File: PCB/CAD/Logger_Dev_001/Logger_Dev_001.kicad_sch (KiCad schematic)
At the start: 11 parts, among them U2 ESP32-C6-WROOM-1

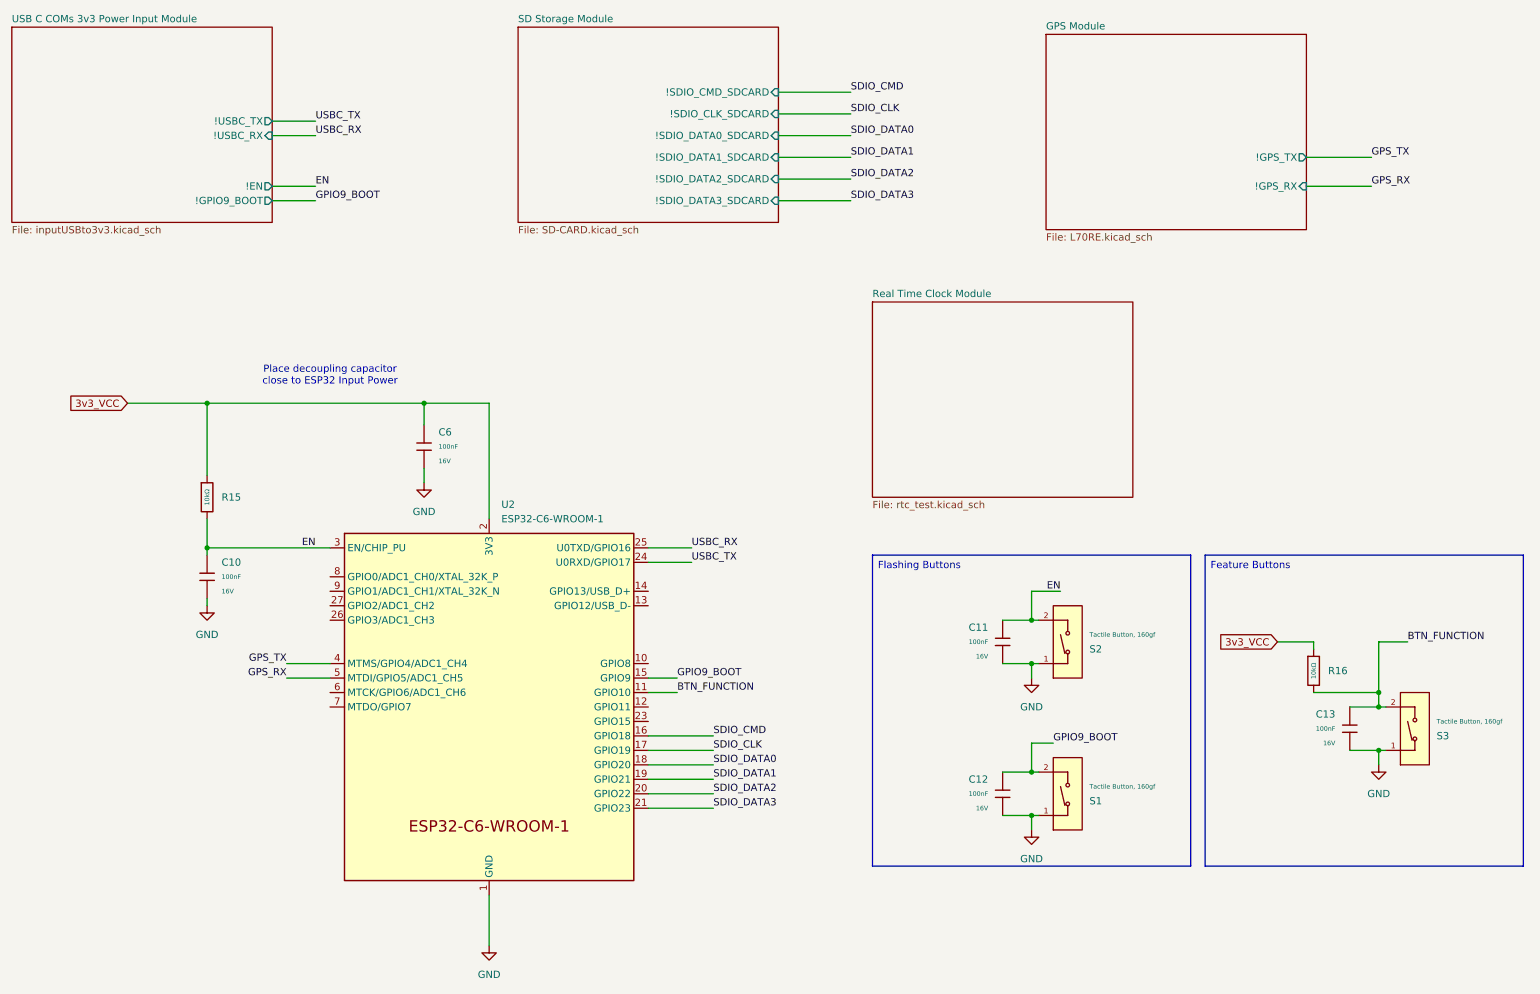
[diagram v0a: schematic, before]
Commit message: Schematic finalised
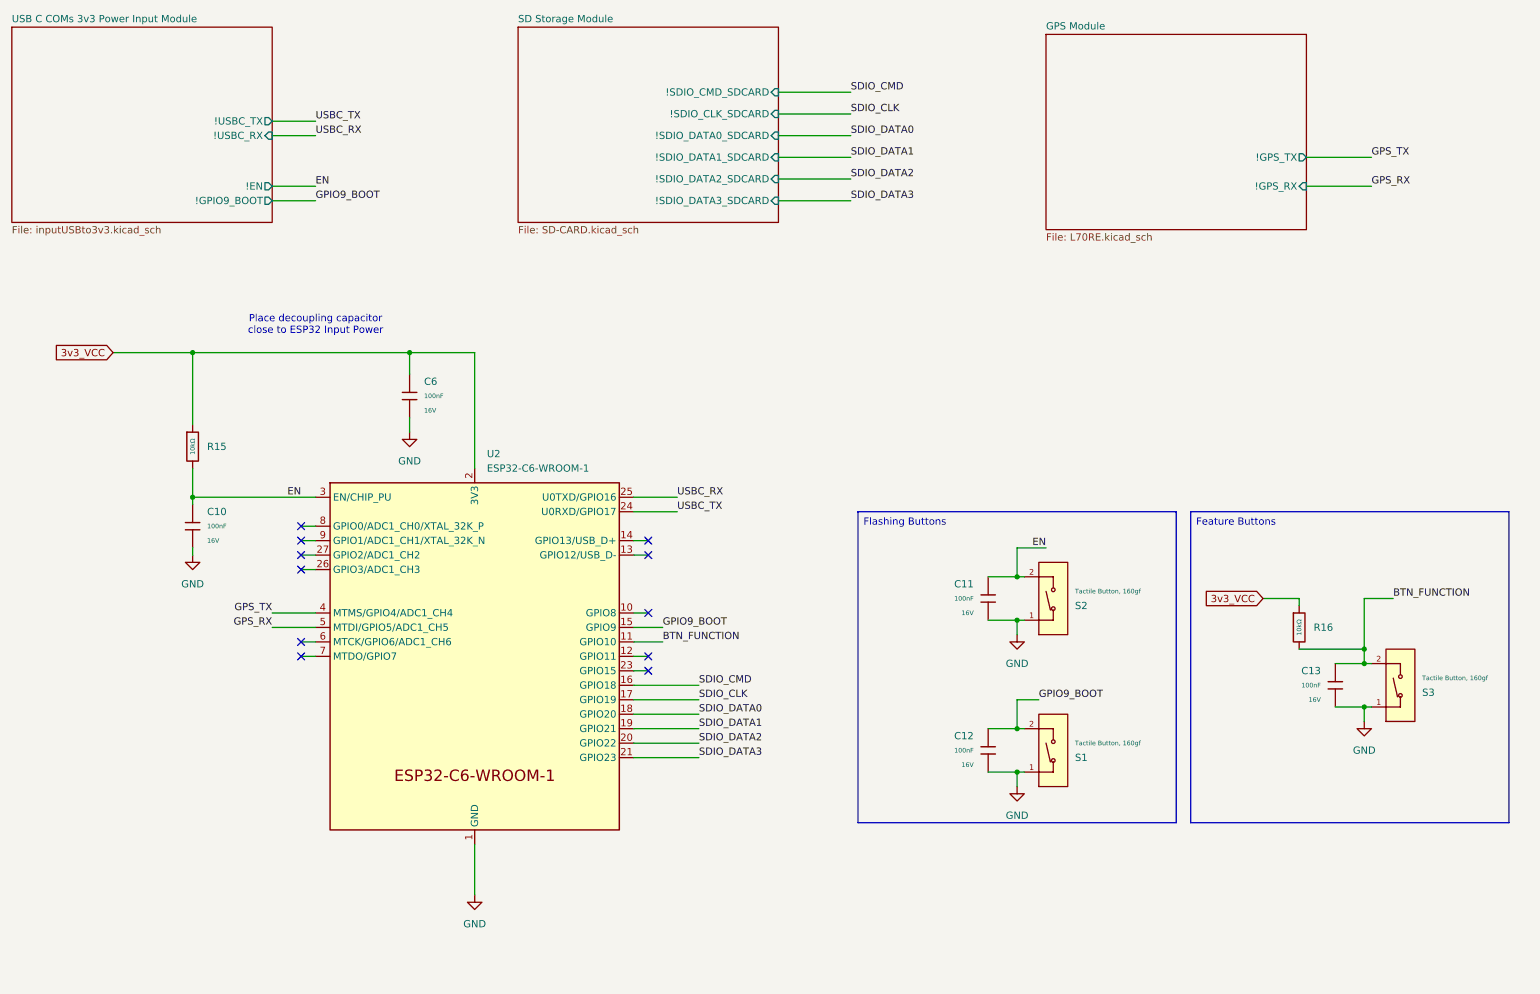
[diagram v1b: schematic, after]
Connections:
- no-connect marks 0 -> 11
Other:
- removed sheet Real Time Clock Module
- moved on the sheet: C10, C11, C12, C13, C6, R15, R16, S1, S2, S3, U2
